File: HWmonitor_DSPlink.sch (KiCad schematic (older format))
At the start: 96 parts, among them J1 USB_B_Mini, J2 Conn_02x04_Odd_Even, T1 760390014, U1 FT232RL, U10 OPA197xDBV, U11 OPA197xDBV, U2 ISO7830DWW, U3 ISO7821DWW, U4 SN6501, U5 TL431DBZ, U6 AD5324ARMZ, U7 TLV70450DBVT, U8 OPA197xDBV, U9 OPA197xDBV, X1 Conn_Coaxial, X2 Conn_Coaxial, X3 Conn_Coaxial, X4 Conn_Coaxial

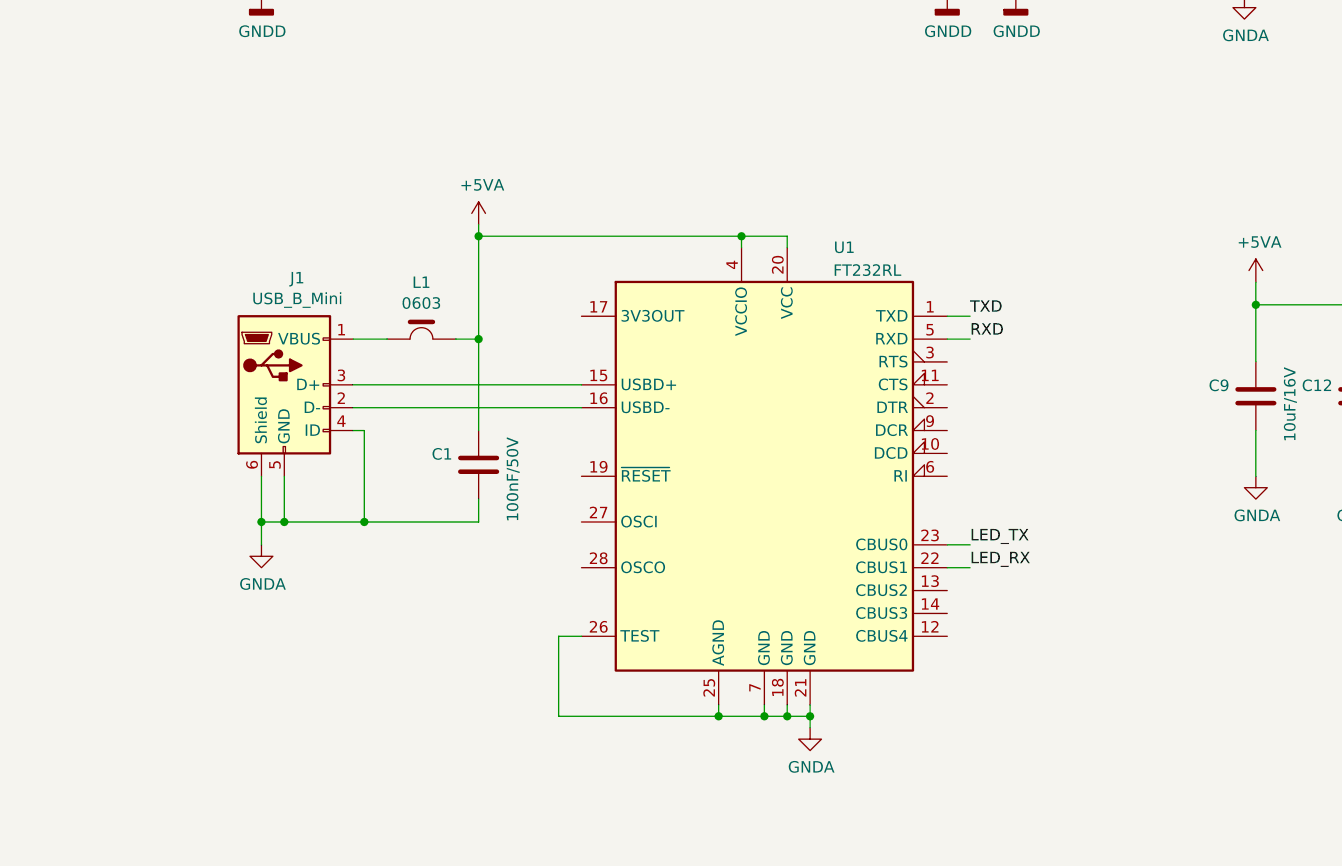
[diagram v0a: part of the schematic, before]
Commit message: placement, added USB input protection
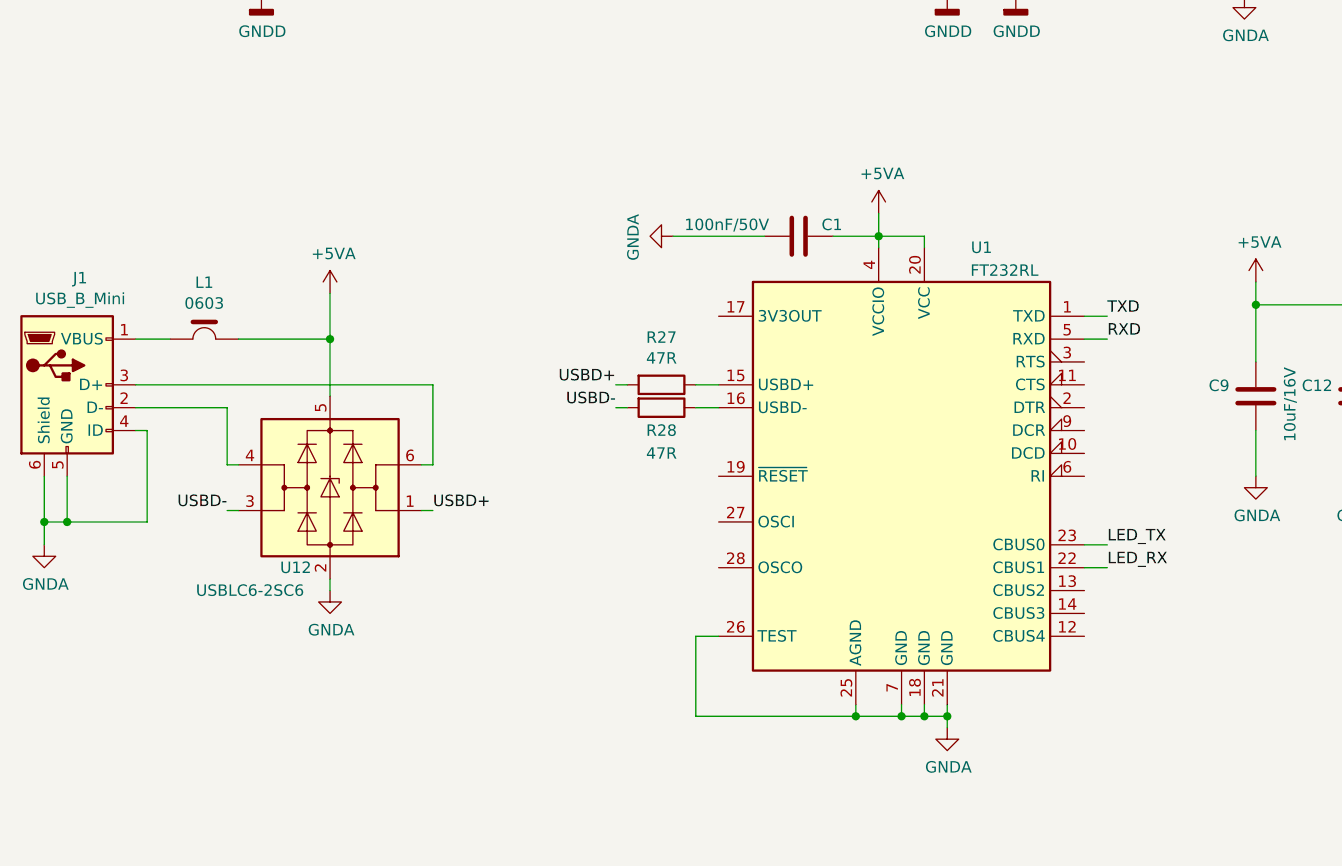
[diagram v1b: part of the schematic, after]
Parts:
- added R27, R28: 47R, Resistor_SMD:R_0603_1608Metric, symbol Device:R
- added U12: USBLC6-2SC6, Package_TO_SOT_SMD:SOT-23-6, symbol Power_Protection:USBLC6-2SC6
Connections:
- net +5VA: now also C1.2, U12.5 (VBUS); no longer C1.1
- net GNDA: now also C1.1, U12.2 (GND); no longer C1.2
- net at U1.15 (USBD+): now also R27.1; no longer J1.3 (D+)
- net at U1.16 (USBD-): now also R28.1; no longer J1.2 (D-)
- new net: J1.2 (D-), U12.4 (I/O2)
- new net: J1.3 (D+), U12.6 (I/O1)
- new net USBD+: R27.2, U12.1 (I/O1)
- new net USBD-: R28.2, U12.3 (I/O2)
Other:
- moved on the sheet: C1, J1, L1, U1
